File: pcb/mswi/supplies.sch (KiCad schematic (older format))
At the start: 11 parts, among them U501 LM7805

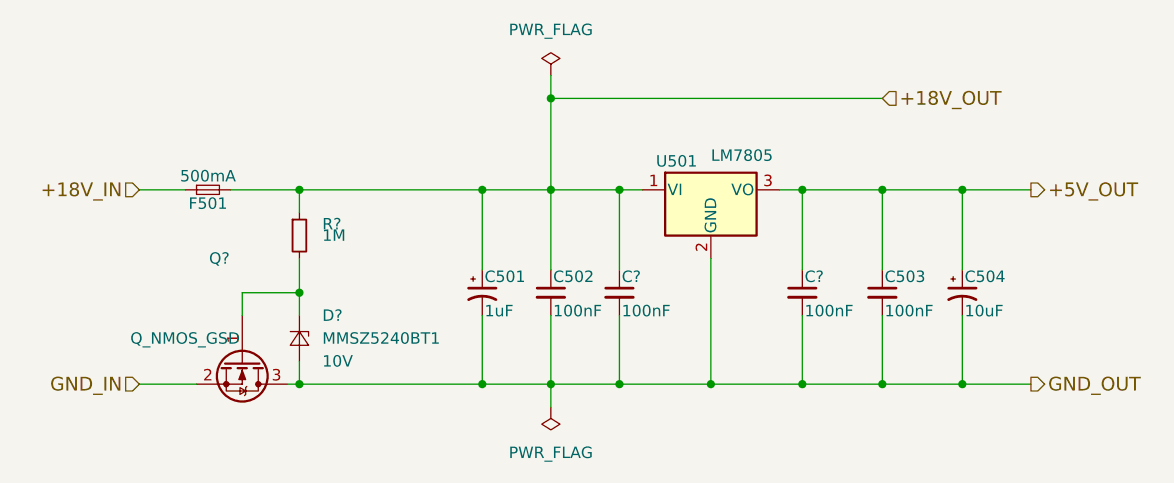
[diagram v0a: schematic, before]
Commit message: Schematics Annotated
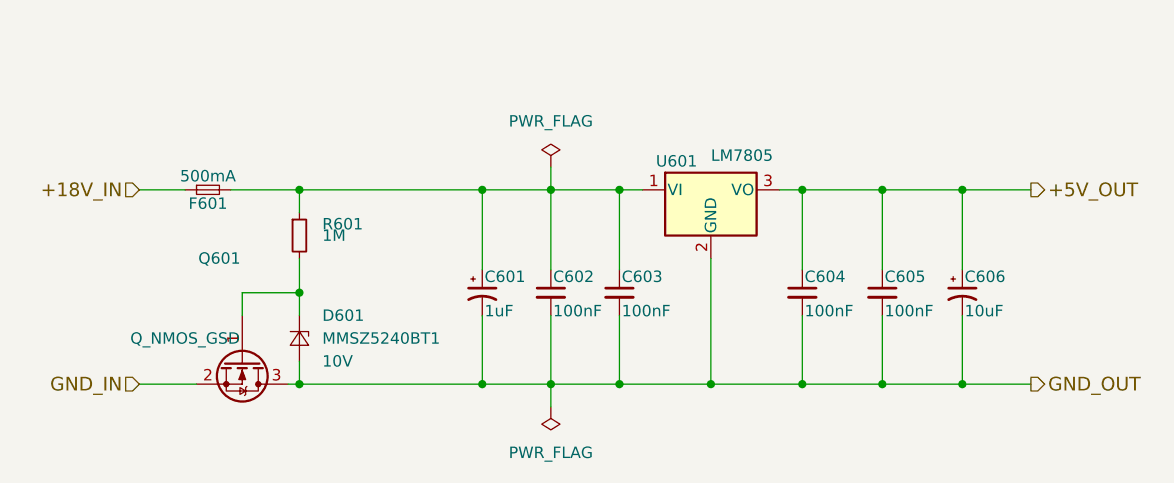
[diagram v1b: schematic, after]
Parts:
- gave numbers to parts that had none: 5
- renumbered C501 to C601, C502 to C602, C503 to C605, C504 to C606, F501 to F601, U501 to U601
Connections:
- net +18V_OUT: no longer names the net of C601.1, C602.1, C603.1, F601.2, R601.1, U601.1 (VI)
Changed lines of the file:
@@
 $Descr A4 11693 8268
 encoding utf-8
-Sheet 4 6
+Sheet 6 6
 Title ""
 Date ""
@@
 $EndDescr
 $Comp
-L Regulator_Linear:LM7805_TO220 U501
+L Regulator_Linear:LM7805_TO220 U601
 U 1 1 5A007B62
 P 5900 3950
-AR Path="/5AACFFEF/5A007B62" Ref="U501"  Part="1"
+AR Path="/5AACFFEF/5A007B62" Ref="U601"  Part="1"
 AR Path="/5DDD6AD9/5A007B62" Ref="U?"  Part="1"
 AR Path="/5DDDDD89/5A007B62" Ref="U?"  Part="1"
-F 0 "U?" H 5750 4075 50  0000 C CNN
+F 0 "U601" H 5750 4075 50  0000 C CNN
 F 1 "LM7805" H 5900 4100 50  0000 L CNN
 F 2 "KicadZeniteSolarLibrary18:TO-220-3_Horizontal_TabDown_SMD" H 5900 4175 50  0001 C CIN
@@
 +5V_OUT
 $Comp
-L Device:CP1_Small C501
+L Device:CP1_Small C601
 U 1 1 5A008895
 P 4900 4400
-AR Path="/5AACFFEF/5A008895" Ref="C501"  Part="1"
+AR Path="/5AACFFEF/5A008895" Ref="C601"  Part="1"
 AR Path="/5DDD6AD9/5A008895" Ref="C?"  Part="1"
 AR Path="/5DDDDD89/5A008895" Ref="C?"  Part="1"
-F 0 "C?" H 4910 4470 50  0000 L CNN
+F 0 "C601" H 4910 4470 50  0000 L CNN
 F 1 "1uF" H 4910 4320 50  0000 L CNN
 F 2 "Capacitor_Tantalum_SMD:CP_EIA-6032-20_AVX-F_Pad2.25x2.35mm_HandSolder" H 4900 4400 50  0001 C CNN
@@
 $EndComp
 $Comp
-L Device:C_Small C502
+L Device:C_Small C602
 U 1 1 5A00899A
 P 5200 4400
-AR Path="/5AACFFEF/5A00899A" Ref="C502"  Part="1"
+AR Path="/5AACFFEF/5A00899A" Ref="C602"  Part="1"
 AR Path="/5DDD6AD9/5A00899A" Ref="C?"  Part="1"
 AR Path="/5DDDDD89/5A00899A" Ref="C?"  Part="1"
-F 0 "C?" H 5210 4470 50  0000 L CNN
+F 0 "C602" H 5210 4470 50  0000 L CNN
 F 1 "100nF" H 5210 4320 50  0000 L CNN
 F 2 "Capacitor_SMD:C_0805_2012Metric_Pad1.15x1.40mm_HandSolder" H 5200 4400 50  0001 C CNN
@@
 +18V_IN
 $Comp
-L Device:C_Small C503
+L Device:C_Small C605
 U 1 1 5A00B18A
 P 6650 4400
-AR Path="/5AACFFEF/5A00B18A" Ref="C503"  Part="1"
+AR Path="/5AACFFEF/5A00B18A" Ref="C605"  Part="1"
 AR Path="/5DDD6AD9/5A00B18A" Ref="C?"  Part="1"
 AR Path="/5DDDDD89/5A00B18A" Ref="C?"  Part="1"
-F 0 "C?" H 6660 4470 50  0000 L CNN
+F 0 "C605" H 6660 4470 50  0000 L CNN
 F 1 "100nF" H 6660 4320 50  0000 L CNN
 F 2 "Capacitor_SMD:C_0805_2012Metric_Pad1.15x1.40mm_HandSolder" H 6650 4400 50  0001 C CNN
@@
 $EndComp
 $Comp
-L Device:CP1_Small C504
+L Device:CP1_Small C606
 U 1 1 5AAD0D5C
 P 7000 4400
-AR Path="/5AACFFEF/5AAD0D5C" Ref="C504"  Part="1"
+AR Path="/5AACFFEF/5AAD0D5C" Ref="C606"  Part="1"
 AR Path="/5DDD6AD9/5AAD0D5C" Ref="C?"  Part="1"
 AR Path="/5DDDDD89/5AAD0D5C" Ref="C?"  Part="1"
-F 0 "C?" H 7010 4470 50  0000 L CNN
+F 0 "C606" H 7010 4470 50  0000 L CNN
 F 1 "10uF" H 7010 4320 50  0000 L CNN
 F 2 "Capacitor_Tantalum_SMD:CP_EIA-6032-20_AVX-F_Pad2.25x2.35mm_HandSolder" H 7000 4400 50  0001 C CNN
@@
 $EndComp
 $Comp
-L Device:Fuse_Small F501
+L Device:Fuse_Small F601
 U 1 1 5AB12173
 P 3700 3950
-AR Path="/5AACFFEF/5AB12173" Ref="F501"  Part="1"
+AR Path="/5AACFFEF/5AB12173" Ref="F601"  Part="1"
 AR Path="/5DDD6AD9/5AB12173" Ref="F?"  Part="1"
 AR Path="/5DDDDD89/5AB12173" Ref="F?"  Part="1"
-F 0 "F?" H 3700 3890 50  0000 C CNN
+F 0 "F601" H 3700 3890 50  0000 C CNN
 F 1 "500mA" H 3700 4010 50  0000 C CNN
 F 2 "Fuse:Fuse_1206_3216Metric_Pad1.42x1.75mm_HandSolder" H 3700 3950 50  0001 C CNN
@@
 Wire Wire Line
 	6650 3950 6650 4300
-Text HLabel 6650 3550 2    60   Input ~ 0
-+18V_OUT
-Wire Wire Line
-	5200 3550 5200 3950
-Wire Wire Line
-	5200 3550 6650 3550
-Connection ~ 5200 3550
-Wire Wire Line
-	5200 3450 5200 3550
-$Comp
-L power:PWR_FLAG #FLG0501
+$Comp
+L power:PWR_FLAG #FLG0601
 U 1 1 5BE75359
-P 5200 3450
-AR Path="/5AACFFEF/5BE75359" Ref="#FLG0501"  Part="1"
+P 5200 3850
+AR Path="/5AACFFEF/5BE75359" Ref="#FLG0601"  Part="1"
 AR Path="/5DDD6AD9/5BE75359" Ref="#FLG?"  Part="1"
 AR Path="/5DDDDD89/5BE75359" Ref="#FLG?"  Part="1"
-F 0 "#FLG?" H 5200 3525 50  0001 C CNN
-F 1 "PWR_FLAG" H 5200 3650 50  0000 C CNN
-F 2 "" H 5200 3450 50  0001 C CNN
-F 3 "~" H 5200 3450 50  0001 C CNN
-	1    5200 3450
-	1    0    0    -1
-$EndComp
-$Comp
-L power:PWR_FLAG #FLG0502
+F 0 "#FLG0601" H 5200 3925 50  0001 C CNN
+F 1 "PWR_FLAG" H 5200 4050 50  0000 C CNN
+F 2 "" H 5200 3850 50  0001 C CNN
+F 3 "~" H 5200 3850 50  0001 C CNN
+	1    5200 3850
+	1    0    0    -1
+$EndComp
+$Comp
+L power:PWR_FLAG #FLG0602
 U 1 1 5BE753AF
 P 5200 4900
-AR Path="/5AACFFEF/5BE753AF" Ref="#FLG0502"  Part="1"
+AR Path="/5AACFFEF/5BE753AF" Ref="#FLG0602"  Part="1"
 AR Path="/5DDD6AD9/5BE753AF" Ref="#FLG?"  Part="1"
 AR Path="/5DDDDD89/5BE753AF" Ref="#FLG?"  Part="1"
-F 0 "#FLG?" H 5200 4975 50  0001 C CNN
+F 0 "#FLG0602" H 5200 4975 50  0001 C CNN
 F 1 "PWR_FLAG" H 5200 5100 50  0000 C CNN
 F 2 "" H 5200 4900 50  0001 C CNN
@@
 	4050 4800 4100 4800
 $Comp
-L Device:Q_NMOS_GSD Q?
+L Device:Q_NMOS_GSD Q601
 U 1 1 5D9E3E7E
 P 3850 4700
-AR Path="/5AACFFEF/5D9E3E7E" Ref="Q?"  Part="1"
+AR Path="/5AACFFEF/5D9E3E7E" Ref="Q601"  Part="1"
 AR Path="/5DDD6AD9/5D9E3E7E" Ref="Q?"  Part="1"
 AR Path="/5DDDDD89/5D9E3E7E" Ref="Q?"  Part="1"
-F 0 "Q?" V 3400 4600 50  0000 C CNN
+F 0 "Q601" V 3400 4600 50  0000 C CNN
 F 1 "Q_NMOS_GSD" V 3750 4450 50  0000 C CNN
 F 2 "" H 4050 4800 50  0001 C CNN
@@
 	4100 4800 4900 4800
 $Comp
-L Device:R_Small R?
+L Device:R_Small R601
 U 1 1 5D9E9D52
 P 4100 4150
-AR Path="/5AACFFEF/5D9E9D52" Ref="R?"  Part="1"
+AR Path="/5AACFFEF/5D9E9D52" Ref="R601"  Part="1"
 AR Path="/5DDD6AD9/5D9E9D52" Ref="R?"  Part="1"
 AR Path="/5DDDDD89/5D9E9D52" Ref="R?"  Part="1"
-F 0 "R?" H 4200 4200 50  0000 L CNN
+F 0 "R601" H 4200 4200 50  0000 L CNN
 F 1 "1M" H 4200 4150 50  0000 L CNN
 F 2 "" H 4100 4150 50  0001 C CNN
@@
 $EndComp
 $Comp
-L Device:D_Zener_Small D?
+L Device:D_Zener_Small D601
 U 1 1 5D9EA99D
 P 4100 4600
-AR Path="/5AACFFEF/5D9EA99D" Ref="D?"  Part="1"
+AR Path="/5AACFFEF/5D9EA99D" Ref="D601"  Part="1"
 AR Path="/5DDD6AD9/5D9EA99D" Ref="D?"  Part="1"
 AR Path="/5DDDDD89/5D9EA99D" Ref="D?"  Part="1"
-F 0 "D?" V 4000 4700 50  0000 L CNN
+F 0 "D601" V 4000 4700 50  0000 L CNN
 F 1 "MMSZ5240BT1" V 4100 4700 50  0000 L CNN
 F 2 "" V 4100 4600 50  0001 C CNN
@@
 	3400 4800 3650 4800
 $Comp
-L Device:C_Small C?
+L Device:C_Small C603
 U 1 1 5D9EFA18
 P 5500 4400
-AR Path="/5AACFFEF/5D9EFA18" Ref="C?"  Part="1"
+AR Path="/5AACFFEF/5D9EFA18" Ref="C603"  Part="1"
 AR Path="/5DDD6AD9/5D9EFA18" Ref="C?"  Part="1"
 AR Path="/5DDDDD89/5D9EFA18" Ref="C?"  Part="1"
-F 0 "C?" H 5510 4470 50  0000 L CNN
+F 0 "C603" H 5510 4470 50  0000 L CNN
 F 1 "100nF" H 5510 4320 50  0000 L CNN
 F 2 "Capacitor_SMD:C_0805_2012Metric_Pad1.15x1.40mm_HandSolder" H 5500 4400 50  0001 C CNN
@@
 	5500 4800 5900 4800
 $Comp
-L Device:C_Small C?
+L Device:C_Small C604
 U 1 1 5D9F17B7
 P 6300 4400
-AR Path="/5AACFFEF/5D9F17B7" Ref="C?"  Part="1"
+AR Path="/5AACFFEF/5D9F17B7" Ref="C604"  Part="1"
 AR Path="/5DDD6AD9/5D9F17B7" Ref="C?"  Part="1"
 AR Path="/5DDDDD89/5D9F17B7" Ref="C?"  Part="1"
-F 0 "C?" H 6310 4470 50  0000 L CNN
+F 0 "C604" H 6310 4470 50  0000 L CNN
 F 1 "100nF" H 6310 4320 50  0000 L CNN
 F 2 "Capacitor_SMD:C_0805_2012Metric_Pad1.15x1.40mm_HandSolder" H 6300 4400 50  0001 C CNN
@@
 Wire Wire Line
 	6300 4800 6650 4800
+Wire Wire Line
+	5200 3850 5200 3950
 $EndSCHEMATC
